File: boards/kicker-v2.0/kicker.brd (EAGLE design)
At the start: 92 x 62 mm, 65 parts, among them J1 B2PS-CENTERED-VH(LF)(SN), J2 B2PS-CENTERED-VH(LF)(SN), J3 B2PS-CENTERED-VH(LF)(SN), J4 HFW8R-1ST, J5 B2PS-CENTERED-VH(LF)(SN), J6 B2PS-CENTERED-VH(LF)(SN), Q1 BUK7Y38-100E, Q2 FDV303N, Q3 FQT1N80, Q4 IXFIXFT94N30P3, Q5 IXFIXFT94N30P3, Q6 FDV303N, Q7 AOD1N60, Q8 FDV303N, T1 DA203X-ALDA2034, U1 LT3757DFN-10, U2 ATTINY441/841MMH/MMHR, U3 IXDN502D1

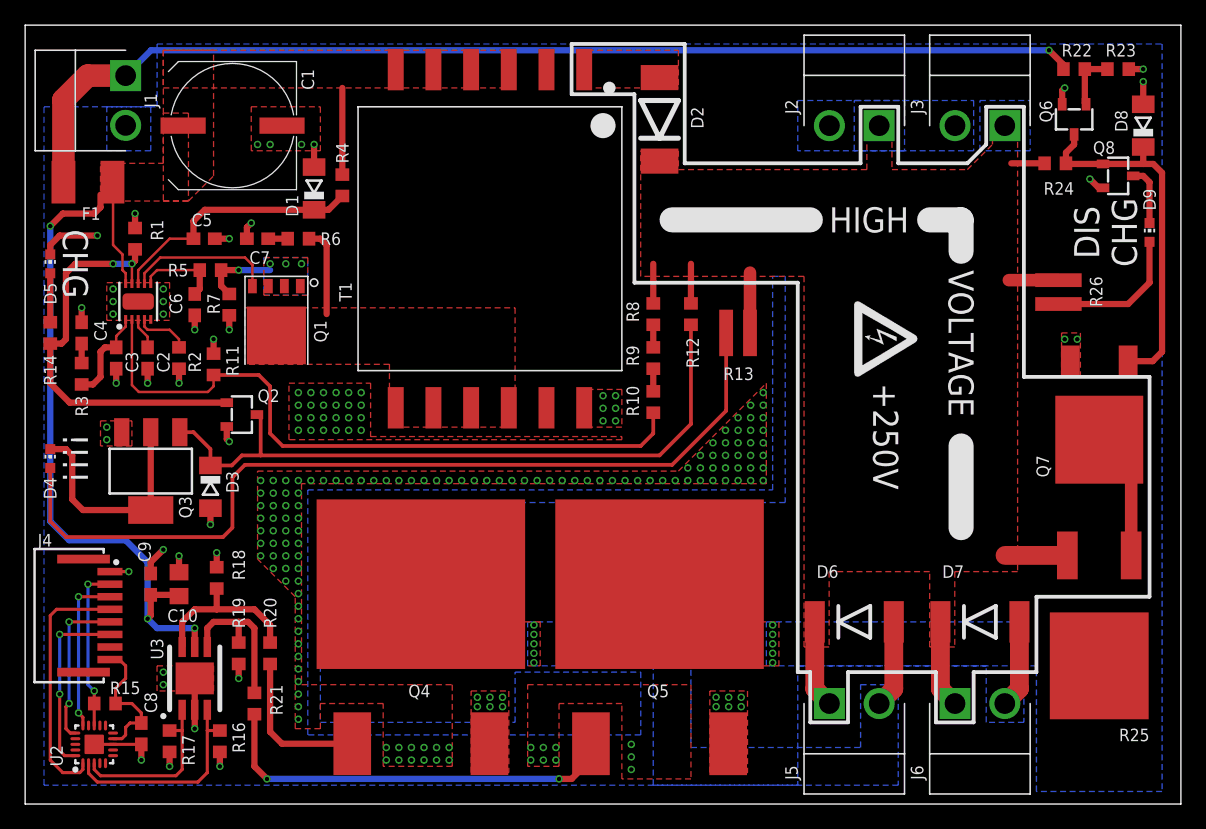
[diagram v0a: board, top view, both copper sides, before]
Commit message: Lots of kicker changes
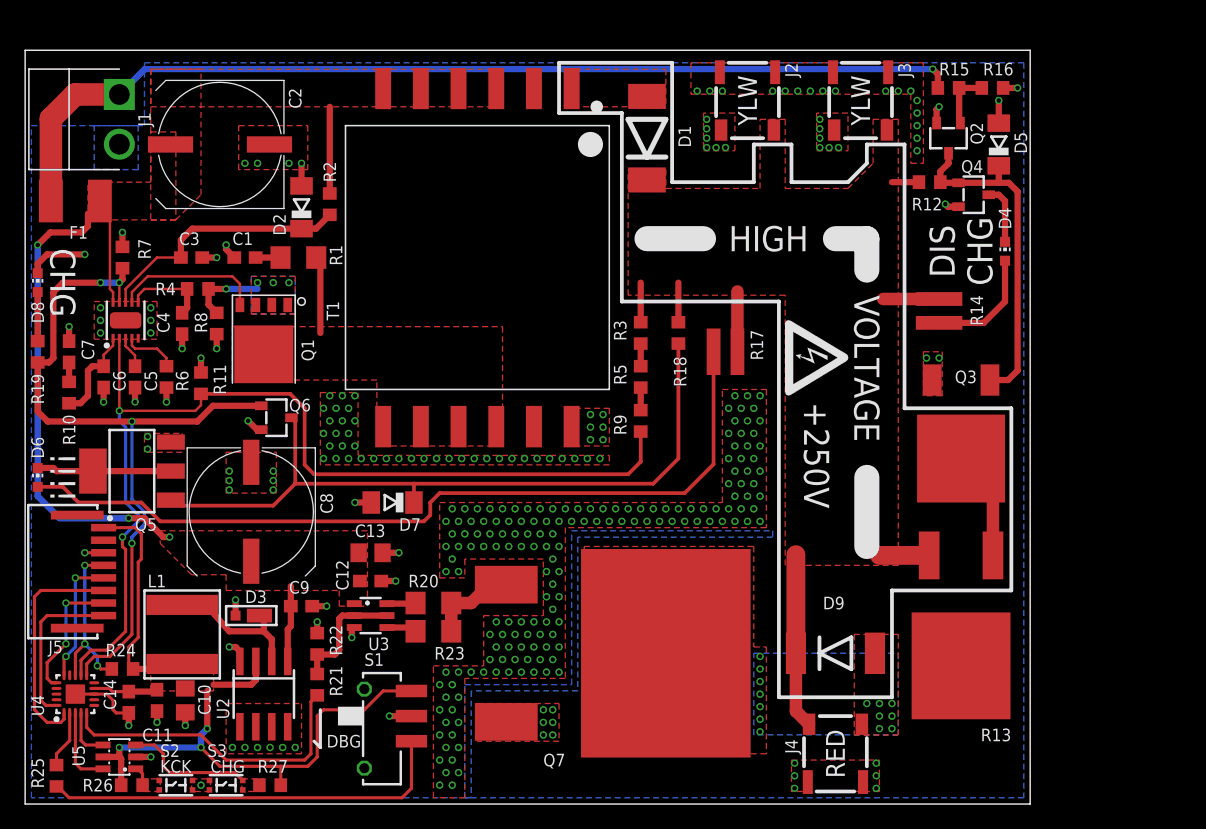
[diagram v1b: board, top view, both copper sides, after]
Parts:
- removed J6: B2PS-CENTERED-VH(LF)(SN), RoboJackets-Connectors:B2PS-CENTERED
- removed Q8: FDV303N, RoboJackets-Discrete:SOT-23-3
- added C11, C12, C14: 0.1uF 35V, rcl:C0603
- added C13: 22uF 35V, rcl:C0805
- added L1: 47uH, RoboJackets-Inductors:NR60XX_NRS60XX
- added R27: 10k, rcl:R0603
- added S1: CSS-121XB, RoboJackets-Switches:CSS-121XB
- added S2, S3: EVPBB2A9B000, RoboJackets-Switches:EVPBB2A9B000
- added U4: ATTINY441/841MMH/MMHR, RoboJackets-ICs:VQFN-20_3X3MM
- added U5: MAX6817, RoboJackets-ICs:SOT-23-6
- C1: value 560uF 25V -> 220pF 100V; device rcl:UD-10X10_NICHICON -> rcl:C0603
- C2: value 0.1uF -> 560uF 25V; device rcl:C0603 -> rcl:UD-10X10_NICHICON
- C3: value 100pF -> 4.7uF 25V
- C5: value 4.7uF 25V -> 0.1uF
- C6: value 0.022uF -> 100pF
- C7: value 220pF 100V -> 0.022uF
- C8: value 0.1uF 35V -> 560uF 25V; device rcl:C0603 -> rcl:UD-10X10_NICHICON
- D1: value BZV55-B18,115 -> ACGRBT30X-HF; device diode:SOD80C -> RoboJackets-Diodes:D2114
- D2: value ACGRBT30X-HF -> BZV55-B18,115; device RoboJackets-Diodes:D2114 -> diode:SOD80C
- D3: value BZV55-B18,115 -> MSS2P3; device diode:SOD80C -> RoboJackets-Diodes:MICROSMP
- D5: value GREEN -> BZV55-B18,115; device RoboJackets-LEDs:CHIP-LED0603 -> diode:SOD80C
- D6: value S10M -> YELLOW; device RoboJackets-Diodes:DO-214AB -> RoboJackets-LEDs:CHIP-LED0603
- D7: value S10M -> BZV55-B18,115; device RoboJackets-Diodes:DO-214AB -> diode:SOD80C
- D8: value BZV55-B18,115 -> GREEN; device diode:SOD80C -> RoboJackets-LEDs:CHIP-LED0603
- D9: value YELLOW -> S10M; device RoboJackets-LEDs:CHIP-LED0603 -> RoboJackets-Diodes:DO-214AB
- J2, J3: value B2PS-CENTERED-VH(LF)(SN) -> SFH-2_RA_L; device RoboJackets-Connectors:B2PS-CENTERED -> RoboJackets-Connectors:SFH-2_RA_L
- J4: value HFW8R-1ST -> SFH-2_RA_R; device RoboJackets-Connectors:HFW8R-1ST -> RoboJackets-Connectors:SFH-2_RA_R
- J5: value B2PS-CENTERED-VH(LF)(SN) -> HFW8R-1ST; device RoboJackets-Connectors:B2PS-CENTERED -> RoboJackets-Connectors:HFW8R-1ST
- Q3: value FQT1N80 -> AOD1N60; device RoboJackets-Discrete:SOT223 -> RoboJackets-Discrete:DPAK
- Q4: value IXFIXFT94N30P3 -> FDV303N; device RoboJackets-Discrete:TO-268 -> RoboJackets-Discrete:SOT-23-3
- Q5: value IXFIXFT94N30P3 -> FQT1N80; device RoboJackets-Discrete:TO-268 -> RoboJackets-Discrete:SOT223
- Q7: value AOD1N60 -> IXFIXFT94N30P3; device RoboJackets-Discrete:DPAK -> RoboJackets-Discrete:TO-268
- R1: value 10k -> 22; device rcl:R0603 -> rcl:R1206
- R10: value 470k 1% -> 6.8k
- R13: value 68k 1W -> 2.5k 35W; device RoboJackets-Resistors:R0612 -> RoboJackets-Resistors:DPAK_TDH
- R14, R17: value 10k -> 68k 1W; device rcl:R0603 -> RoboJackets-Resistors:R0612
- R15: value 10k -> 270k
- R16: value 10k -> 100k
- R18: value 10k -> 10M
- R20: value 2k -> 22; device rcl:R0603 -> rcl:R1206
- R21: value 2k -> 500
- R22: value 270k -> 10k
- R23: value 100k -> 22; device rcl:R0603 -> rcl:R1206
- R24: value 10M -> 10k
- R25: value 2.5k 35W -> 10k; device RoboJackets-Resistors:DPAK_TDH -> rcl:R0603
- R26: value 68k 1W -> 10k; device RoboJackets-Resistors:R0612 -> rcl:R0603
- R3: value 6.8k -> 1M 1%
- R4: value 140k -> 22
- R5: value 22 -> 1M 1%
- R6: value 22 -> 140k
- R7: value 0.015 -> 10k
- R8: value 1M 1% -> 0.015
- R9: value 1M 1% -> 470k 1%
- U2: value ATTINY441/841MMH/MMHR -> AP1509-50; device RoboJackets-ICs:VQFN-20_3X3MM -> RoboJackets-PowerICs:SOIC-8
- U3: value IXDN502D1 -> ZXGD3003; device RoboJackets-PowerICs:DFN-6_4X5MM -> RoboJackets-PowerICs:SOT-23-6
- moved D8 88.9 mm to (1.00, 41.5), turned to 0 degrees
- moved R24 84.5 mm to (7.75, 10.8), turned to 0 degrees
- moved R26 83.5 mm to (8.50, 1.50), turned to 180 degrees
- moved R25 83.5 mm to (2.50, 2.25), turned to 270 degrees
- moved R15 83.1 mm to (73.5, 57.0), turned to 180 degrees
- moved R16 80.5 mm to (77.0, 57.0), turned to 180 degrees
- moved D4 77.8 mm to (78.0, 44.0)
- moved D5 76.1 mm to (77.5, 52.5), turned to 90 degrees
- moved R22 75.7 mm to (23.2, 12.8), turned to 270 degrees
- moved R14 70.8 mm to (72.8, 39.2), turned to 90 degrees
- moved R23 70.5 mm to (32.5, 13.8), turned to 0 degrees
- moved Q6 67.8 mm to (20.0, 30.8), turned to 270 degrees
- moved D6 66.0 mm to (1.00, 26.0)
- moved Q3 64.5 mm to (74.5, 27.5)
- moved J5 63.9 mm to (3.00, 18.5), turned to 270 degrees
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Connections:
- removed net CHIP: R17.2, U2.3, U3.1
- removed net CHIPPER: D6.A, J5.2, Q4.4
- removed net CHIP_GATE: R18.2, R20.1, U3.6
- removed net KICK_GATE: R19.2, R21.1, U3.4
- new net !CHARGE_BTN: R27.1, S3.B1, S3.B2, U5.3
- new net !CHARGE_BTN_DB: U4.4, U5.4
- new net !KICK_BTN: R26.1, S2.A1, S2.A2, U5.1
- new net !KICK_BTN_DB: U4.3, U5.6
- new net DBG_MODE: R25.1, U4.2
- new net N$14: D3.K, L1.2, U2.2
- new net N$15: R20.1, U3.6
- new net N$16: R23.1, U3.4
- new net N$9: R25.2, S1.3
- net !KICKER_SELECT: now also J5.5, U4.15; no longer J4.3, U2.15
- net !RESET: now also J5.4, R24.1, U4.13; no longer J4.2, R15.1, U2.13
- net +18.5V: now also C12.1, C13.1, C2.+, C8.+, R2.1, U2.1, U3.1; no longer C1.+, C10.1, R4.1, U3.5
- net +5V: now also C10.1, C11.1, C14.1, J5.1, L1.1, R24.2, R26.2, R27.2, S1.1, U2.3, U4.9, U5.5; no longer C8.1, J4.8, R15.2, U2.9
- net CHARGE: now also Q6.1, R19.2, R7.2, U4.11; no longer Q2.1, R1.2, R14.2
- net FB: now also R9.1, U4.12; no longer R10.1
- net GND: now also C1.2, C11.2, C12.2, C13.2, C14.2, C2.-, C8.-, D2.A, D5.A, D7.A, D8.C, J2.LEG1, J2.LEG2, J3.LEG1, J3.LEG2, J4.LEG1, J4.LEG2, J5.3, Q4.2, R22.1, R6.1, R8.1, S1.2, S1.LEG1, S1.LEG4, S2.B1, S2.B2, S3.A1, S3.A2, U2.4, U2.5, U2.6, U2.7, U3.3, U4.8, U4.PAD, U5.2; no longer C1.-, C2.2, C8.2, D1.A, D5.C, D8.A, J4.1, Q4.3, Q8.2, R1.1, R17.1, R18.1, R19.1, R2.1, R23.1, U2.PAD, U3.2, U3.PAD
- net HV_AC: now also D1.A; no longer D2.A
- net INTVCC: now also C3.1, D2.C, R2.2; no longer C5.1, D1.C, R4.2
- net KICK: now also R21.1, U4.5; no longer R16.2, U2.2, U3.3
- net KICKER: now also D9.A, J4.2, Q7.4; no longer D7.A, J6.2, Q5.4
- net MISO: now also J5.8, U4.20; no longer J4.6, U2.20
- net MOSI: now also J5.7, U4.16; no longer J4.5, U2.16
- net N$1: now also C7.1, R10.2; no longer C4.1, R3.2
- net N$10: now also Q2.1, R15.1, R16.2; no longer Q6.1, R22.1, R23.2
- net N$11: now also D4.C, Q4.3; no longer D9.C, Q8.3
- net N$12: now also Q3.FIN, R13.1; no longer Q7.FIN, R25.1
- net N$13: now also D4.A, R14.1; no longer D9.A, R26.1
- net N$2: now also C6.1, R10.1; no longer C3.1, R3.1
- net N$21: now also D7.C, Q5.1, Q6.3, R18.1; no longer D3.C, Q2.3, Q3.1, R12.1
- net N$3: now also D6.A, R17.1; no longer D4.A, R13.1
- net N$32: now also C1.1, R1.1; no longer C7.1, R6.1
- net N$4: now also D6.C, Q5.2, Q5.4; no longer D4.C, Q3.2, Q3.4
- net N$5: now also D8.A, R19.1; no longer D5.A, R14.1
- net N$7: now also R21.2, R22.2, U3.2, U3.5; no longer Q4.1, R20.2
- net N$8: now also Q7.1, R20.2, R23.2; no longer Q5.1, R21.2
- net QUICK_DISCHARGE: now also D5.C, Q2.3, Q3.1, Q4.1, R12.1; no longer D8.C, Q6.3, Q7.1, Q8.1, R24.1
- net RTIMING: now also R6.2; no longer R2.2
- net RTOP12: now also R3.1, R5.2; no longer R8.1, R9.2
- net RTOP23: now also R5.1, R9.2; no longer R10.2, R9.1
- net SCK: now also J5.6, U4.1; no longer J4.4, U2.1
- net SENSE: now also R4.2, R8.2; no longer R5.2, R7.2
- net SENSE_LPF: now also C4.1, R4.1; no longer C6.1, R5.1
- net SOFT-START: now also C5.1; no longer C2.1
- net V+: now also D1.K, D9.C, J4.1, R14.2, R17.2, R18.2, R3.2; no longer D2.K, D6.C, D7.C, J5.1, J6.1, R24.2, R25.2, R26.2, R8.2
- net VBATT: now also R15.2; no longer R22.2
- net VSN: now also R1.2; no longer R6.2
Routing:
- net +5V: track 11.1 -> 64.9 mm, vias 0 -> 3
- net N$9: track 0.00 -> 32.7 mm
- net CHARGE: track 32.9 -> 60.8 mm, vias 2 -> 4
- net FB: track 54.6 -> 81.0 mm, vias 0 -> 2
- net N$8: track 33.3 -> 7.23 mm, vias 2 -> 0
- net CHIP: track 13.7 -> 0.00 mm
- net CHIP_GATE: track 13.0 -> 0.00 mm
- net KICK_GATE: track 12.5 -> 0.00 mm
- net N$14: track 0.00 -> 11.5 mm
- net !CHARGE_BTN: track 0.00 -> 10.3 mm
- net +18.5V: track 66.5 -> 57.1 mm
- net VBATT: track 88.6 -> 80.1 mm
- net KICK: track 16.9 -> 25.1 mm
- net N$4: track 18.3 -> 10.7 mm
- net KICKER: track 6.98 -> 0.00 mm, vias 5 -> 14
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- added copper zone on layer 1, net !CHARGE_BTN
- added copper zone on layer 1, net !KICK_BTN
- added copper zone on layer 1, net +5V
- removed copper zone on layer 1, net CHIPPER
- removed copper zone on layer 16, net CHIPPER
- removed copper zone on layer 16, net N$9
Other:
- board size 92 x 62 mm -> 80 x 60 mm
- board text added: "#"
- board text added: "DBG"
- board text added: "KCK"
- board text added: "RoboCup-SSL Kicker V2.0"
